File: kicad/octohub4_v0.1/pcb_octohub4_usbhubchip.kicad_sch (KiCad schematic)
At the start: 34 parts, among them J301 USB_C_Receptacle_USB2.0, U302 USB2514B_Bi, Y301 24MHz

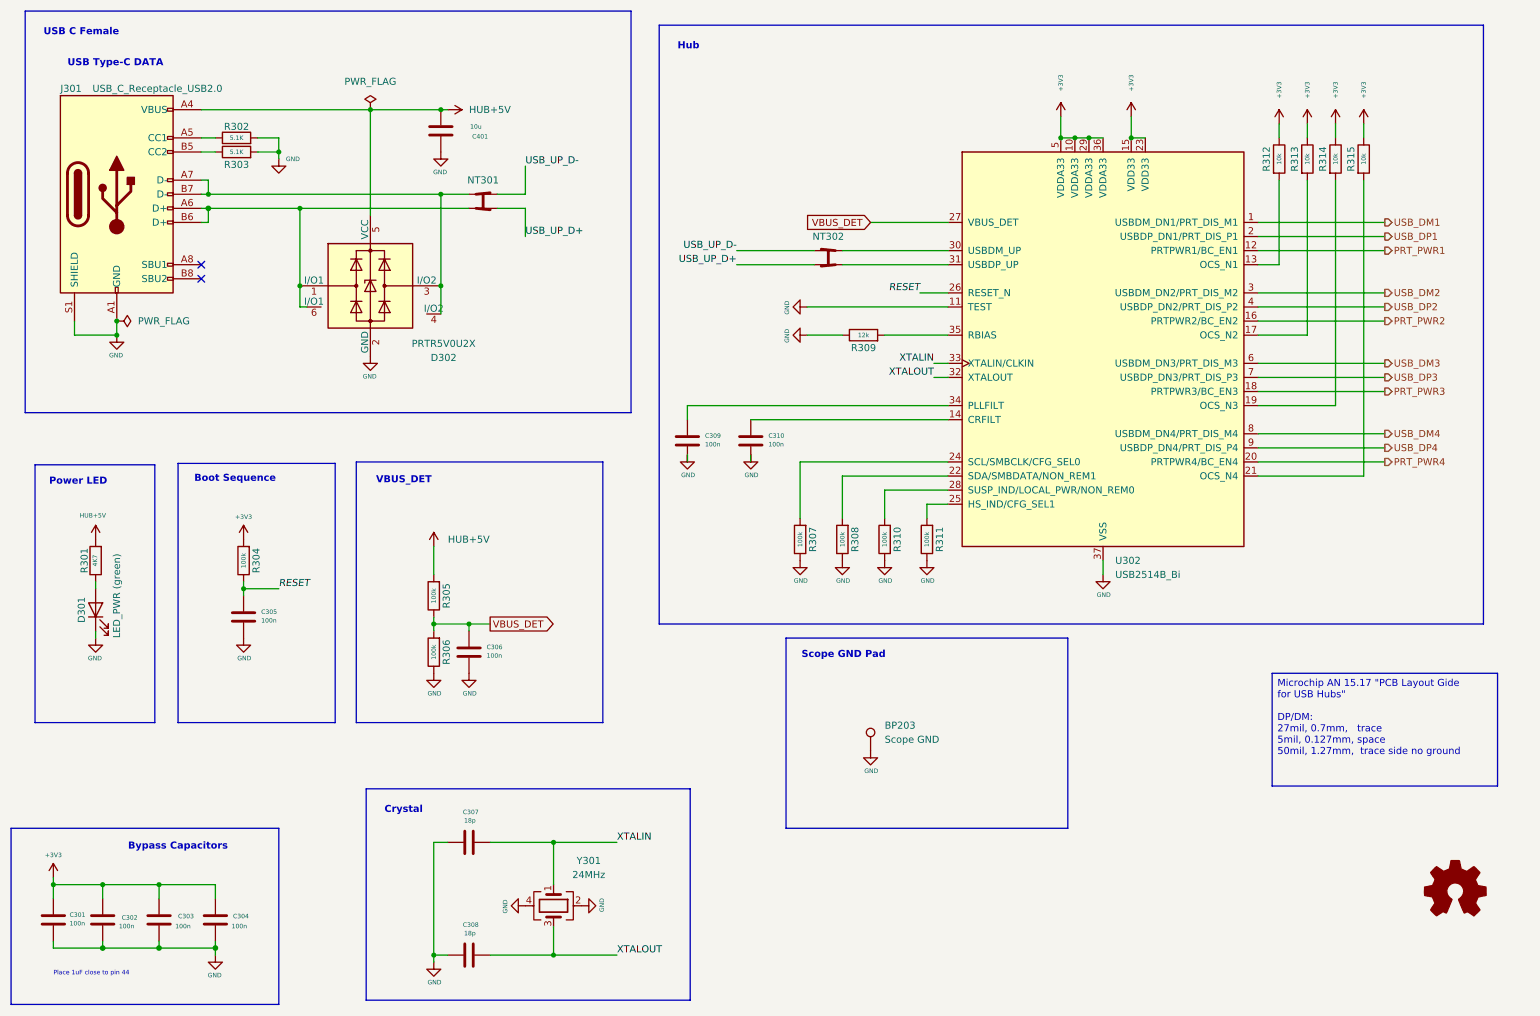
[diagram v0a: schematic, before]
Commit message: tmp
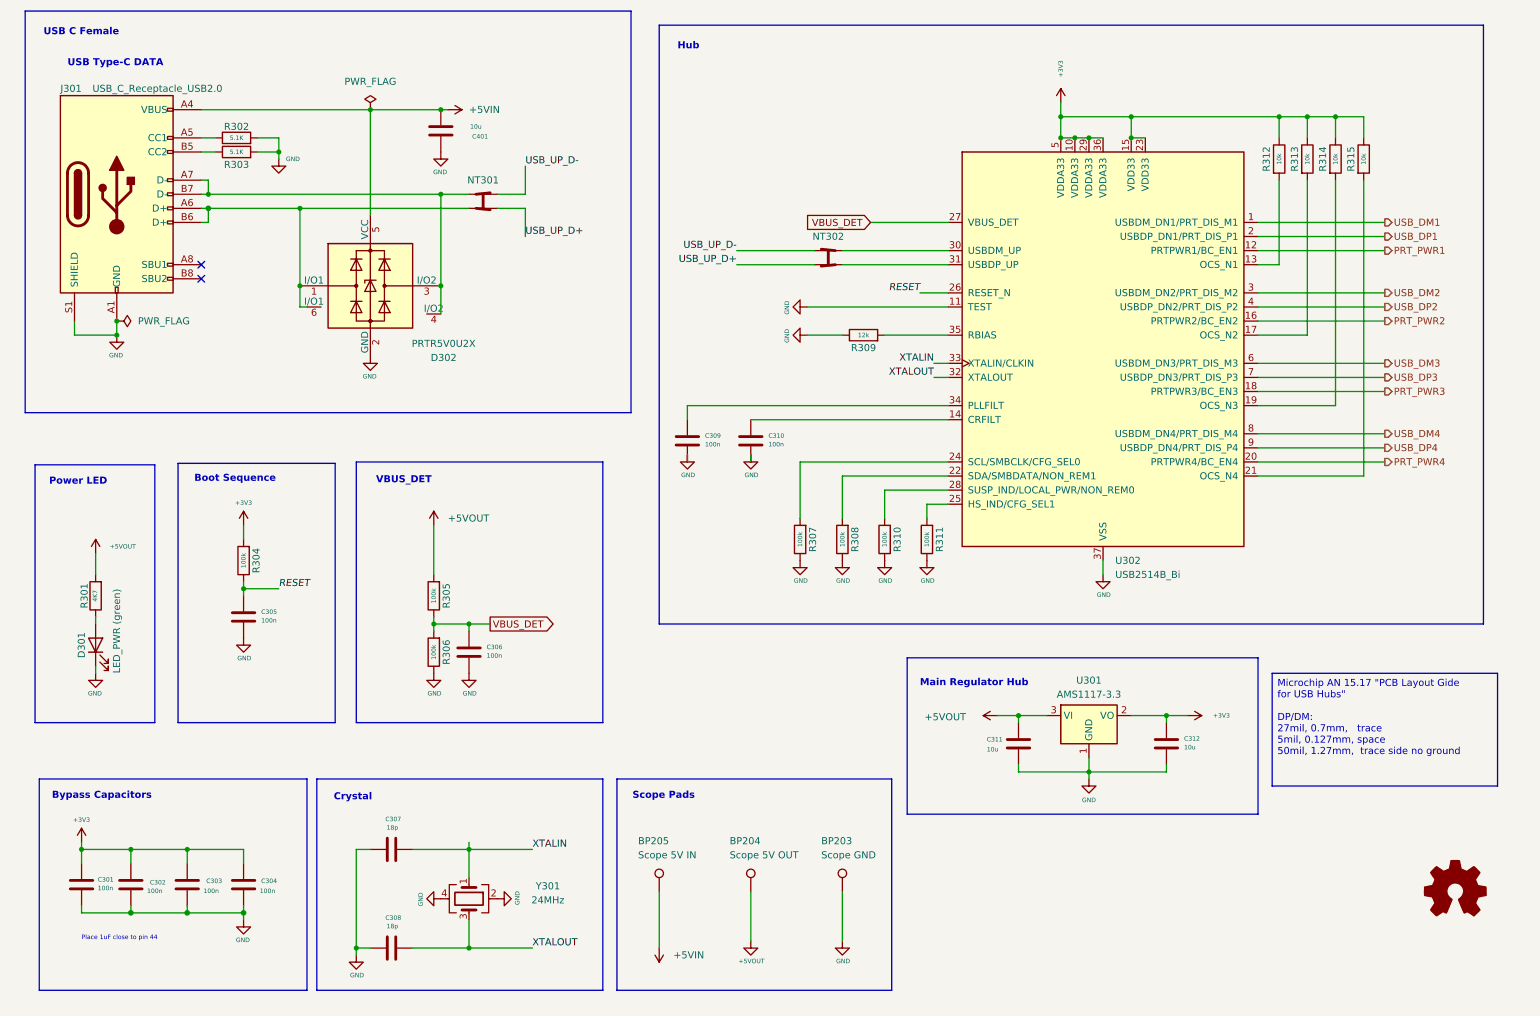
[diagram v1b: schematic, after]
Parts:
- added BP204: Scope 5V OUT, 00_project_library:octoprobe_breakout_PB, symbol 00_project_library:octoprobe_breakout_BP
- added BP205: Scope 5V IN, 00_project_library:octoprobe_breakout_PB, symbol 00_project_library:octoprobe_breakout_BP
- added C311, C312: 10u, Capacitor_SMD:C_0603_1608Metric, symbol 00_project_library:C
- added U301: AMS1117-3.3, 00_project_library:SOT-223-3_TabPin2, symbol 00_project_library:AMS1117-3.3
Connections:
- net +3V3: now also C312.1, U301.2 (VO)
- net GND: now also C311.2, C312.2, U301.1 (GND)
- net HUB+5V renamed +5VIN
- net +5VIN: now also BP205.1; no longer R301.2, R305.2
- new net +5VOUT: BP204.1, C311.1, R301.2, R305.2, U301.3 (VI)
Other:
- note added: "Main Regulator Hub"
- note added: "Scope Pads"
- note removed: "Scope GND Pad"
- moved on the sheet: BP203, C301, C302, C303, C304, C307, C308, D301, R301, Y301
